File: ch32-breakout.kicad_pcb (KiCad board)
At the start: 2 copper layers, 18 x 35.5 mm, 37 parts, among them J1 Conn_ARM_SWD_TagConnect_TC203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, J2 USB_C_Receptacle_USB2.0_16P, J3 Conn_01x05_Socket, J4 Conn_01x05_Socket, J5 Conn_01x05_Socket, J6 Conn_01x05_Socket, Q1 Q_Dual_PMOS_S1G1D2S2G2D1, U1 CH32V003FxUx, U2 TP4057, U3 XB3303ASOT23, U4 XC6206PxxxMR

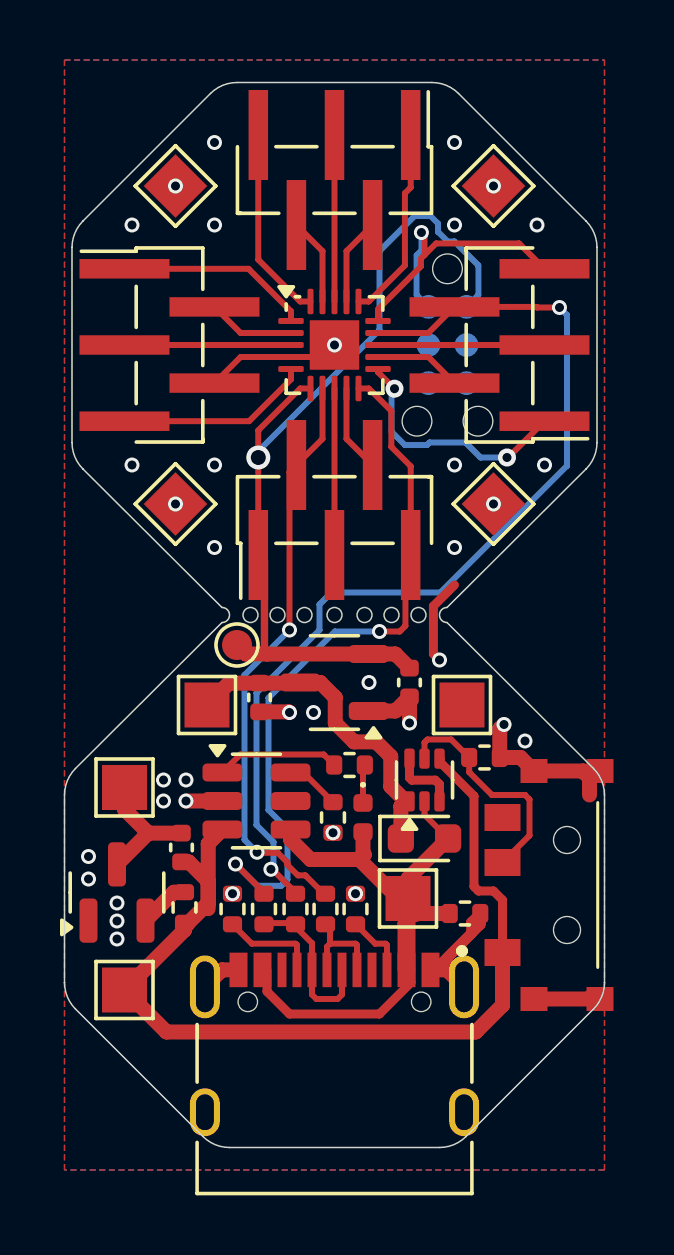
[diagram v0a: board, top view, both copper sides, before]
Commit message: Bpard finished it's kibot time
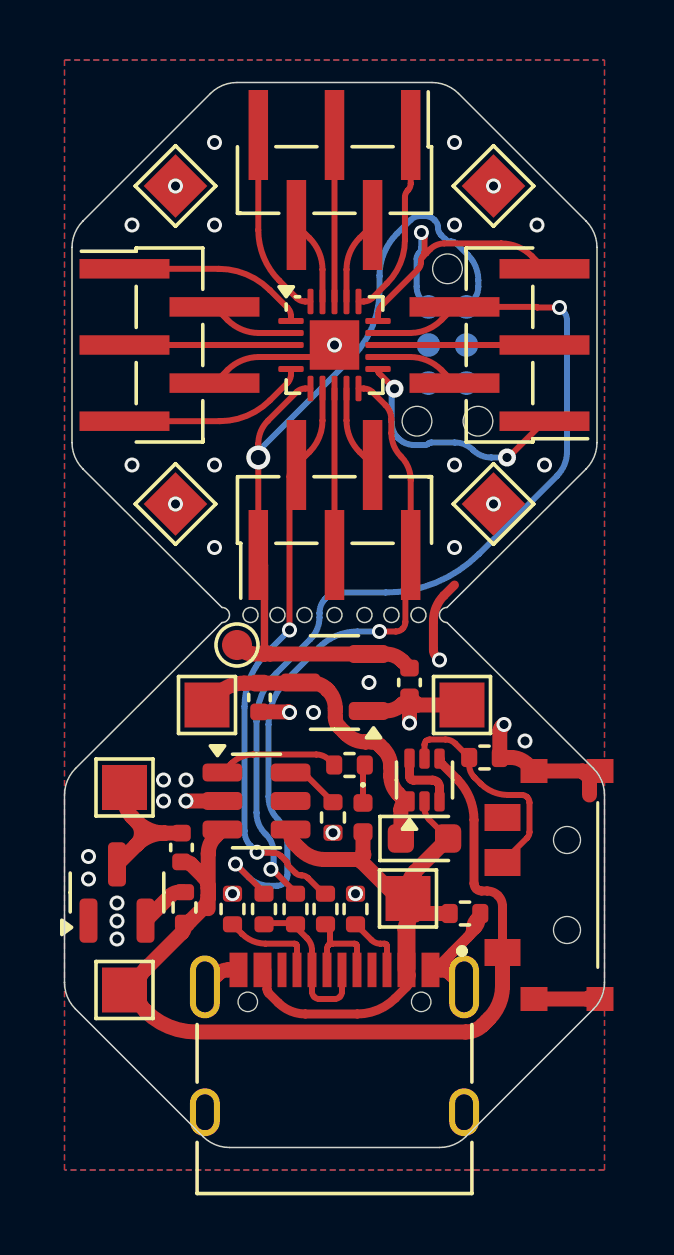
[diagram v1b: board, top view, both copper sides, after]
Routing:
- net Net-(U3-GND): track 4.43 -> 5.66 mm
- net +BATT: track 31.8 -> 30.7 mm
- net DPU: track 33.1 -> 32.4 mm
- net D-: track 24.2 -> 23.7 mm
